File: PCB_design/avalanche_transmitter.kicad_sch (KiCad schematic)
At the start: 22 parts, among them J1 Conn_01x07_Pin, Q1 2N3904, SW1 SW_Push, U1 74HC00

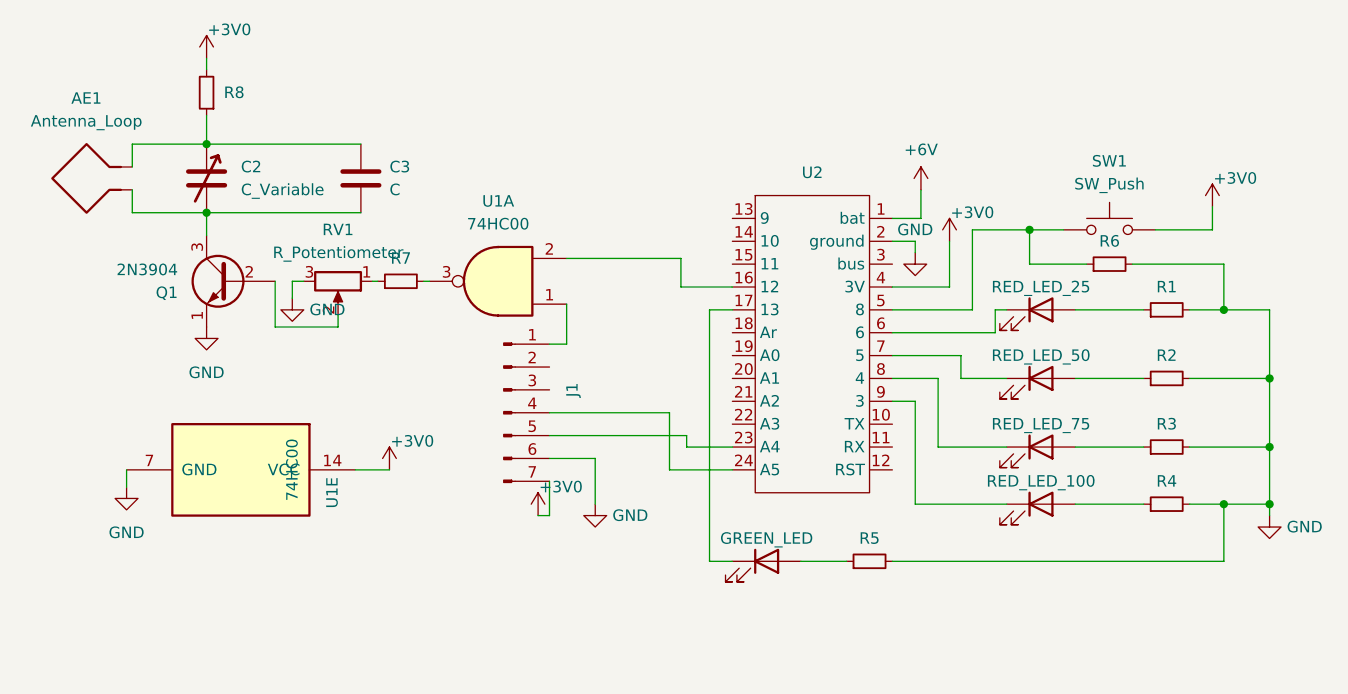
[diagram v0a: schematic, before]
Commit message: Final PCB
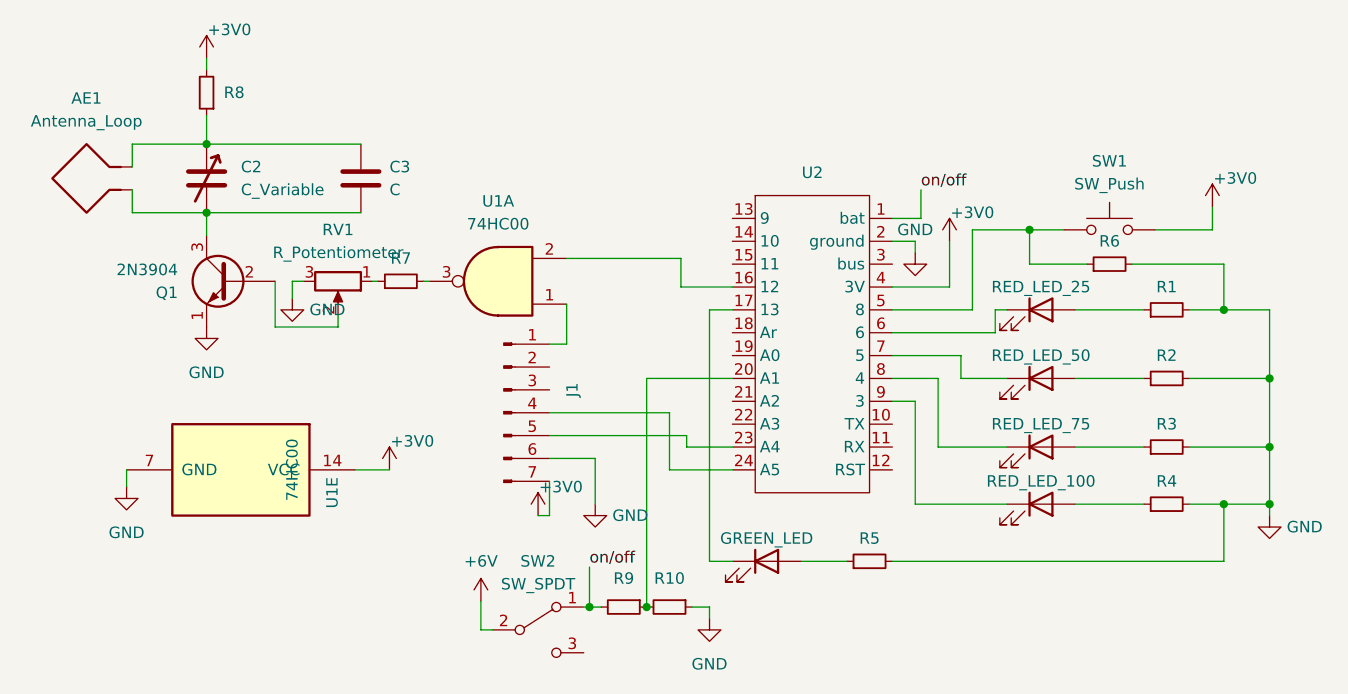
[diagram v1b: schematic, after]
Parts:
- added R10, R9: R_Small, Resistor_THT:R_Axial_DIN0204_L3.6mm_D1.6mm_P7.62mm_Horizontal, symbol Device:R_Small
- added SW2: SW_SPDT, Connector_PinHeader_2.54mm:PinHeader_1x03_P2.54mm_Vertical, symbol Switch:SW_SPDT
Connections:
- net +6V: now also SW2.2 (B); no longer U2.1 (bat)
- net GND: now also R10.1
- net at U2.20 (A1): now also R10.2, R9.1
- new net on/off: R9.2, SW2.1 (A), U2.1 (bat)
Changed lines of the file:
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@@
   (junction (at 196.85 66.04) (diameter 0) (color 0 0 0 0)
   )
+  (junction (at 126.365 77.47) (diameter 0) (color 0 0 0 0)
+  )
   (junction (at 175.26 35.56) (diameter 0) (color 0 0 0 0)
   )
+  (junction (at 132.715 77.47) (diameter 0) (color 0 0 0 0)
+  )
   (junction (at 83.82 26.035) (diameter 0) (color 0 0 0 0)
   )
@@
     (stroke (width 0) (type default))
   )
+  (wire (pts (xy 132.715 52.07) (xy 132.715 77.47))
+    (stroke (width 0) (type default))
+  )
   (wire (pts (xy 167.64 52.07) (xy 167.64 49.53))
     (stroke (width 0) (type default))
@@
     (stroke (width 0) (type default))
   )
+  (wire (pts (xy 126.365 73.025) (xy 126.365 77.47))
+    (stroke (width 0) (type default))
+  )
   (wire (pts (xy 196.85 66.04) (xy 201.93 66.04))
     (stroke (width 0) (type default))
@@
     (stroke (width 0) (type default))
   )
+  (wire (pts (xy 137.795 77.47) (xy 139.7 77.47))
+    (stroke (width 0) (type default))
+  )
   (wire (pts (xy 74.93 62.23) (xy 74.93 64.135))
     (stroke (width 0) (type default))
@@
     (stroke (width 0) (type default))
   )
+  (wire (pts (xy 114.3 76.835) (xy 114.3 80.01))
+    (stroke (width 0) (type default))
+  )
   (wire (pts (xy 136.525 41.91) (xy 142.24 41.91))
     (stroke (width 0) (type default))
@@
     (stroke (width 0) (type default))
   )
+  (wire (pts (xy 142.24 52.07) (xy 132.715 52.07))
+    (stroke (width 0) (type default))
+  )
   (wire (pts (xy 107.95 41.275) (xy 108.585 41.275))
     (stroke (width 0) (type default))
   )
+  (wire (pts (xy 139.7 77.47) (xy 139.7 78.74))
+    (stroke (width 0) (type default))
+  )
   (wire (pts (xy 137.16 59.69) (xy 142.24 59.69))
     (stroke (width 0) (type default))
@@
     (stroke (width 0) (type default))
   )
+  (wire (pts (xy 125.73 77.47) (xy 126.365 77.47))
+    (stroke (width 0) (type default))
+  )
   (wire (pts (xy 171.45 46.99) (xy 160.02 46.99))
     (stroke (width 0) (type default))
@@
     (stroke (width 0) (type default))
   )
+  (wire (pts (xy 114.3 80.01) (xy 115.57 80.01))
+    (stroke (width 0) (type default))
+  )
   (wire (pts (xy 75.565 31.115) (xy 75.565 33.655))
     (stroke (width 0) (type default))
@@
     (stroke (width 0) (type default))
   )
+  (wire (pts (xy 126.365 77.47) (xy 127.635 77.47))
+    (stroke (width 0) (type default))
+  )
   (wire (pts (xy 180.34 44.45) (xy 187.96 44.45))
     (stroke (width 0) (type default))
@@
   (wire (pts (xy 135.255 62.23) (xy 142.24 62.23))
     (stroke (width 0) (type default))
+  )
+  (label "on{slash}off" (at 163.195 31.115 0) (fields_autoplaced)
+    (effects (font (size 1.27 1.27)) (justify left bottom))
+  )
+  (label "on{slash}off" (at 126.365 73.025 0) (fields_autoplaced)
+    (effects (font (size 1.27 1.27)) (justify left bottom))
   )
   (symbol (lib_id "Device:R_Small") (at 83.82 20.32 180) (unit 1)
@@
     )
   )
+  (symbol (lib_id "Switch:SW_SPDT") (at 120.65 80.01 0) (unit 1)
+    (in_bom yes) (on_board yes) (dnp no) (fields_autoplaced)
+    (property "Reference" "SW2" (at 120.65 72.39 0)
+      (effects (font (size 1.27 1.27)))
+    )
+    (property "Value" "SW_SPDT" (at 120.65 74.93 0)
+      (effects (font (size 1.27 1.27)))
+    )
+    (property "Footprint" "Connector_PinHeader_2.54mm:PinHeader_1x03_P2.54mm_Vertical" (at 120.65 80.01 0)
+      (effects (font (size 1.27 1.27)) hide)
+    )
+    (property "Datasheet" "~" (at 120.65 80.01 0)
+      (effects (font (size 1.27 1.27)) hide)
+    )
+    (pin "1")
+    (pin "2")
+    (pin "3")
+    (instances
+      (project "avalanche_transmitter"
+        (path "/8c884e5d-9429-461a-a115-9f5a3e16f11a"
+          (reference "SW2") (unit 1)
+        )
+      )
+    )
+  )
   (symbol (lib_id "power:+3V0") (at 195.58 33.02 0) (unit 1)
     (in_bom yes) (on_board yes) (dnp no)
@@
         (path "/8c884e5d-9429-461a-a115-9f5a3e16f11a"
           (reference "#PWR09") (unit 1)
+        )
+      )
+    )
+  )
+  (symbol (lib_id "power:+6V") (at 114.3 76.835 0) (unit 1)
+    (in_bom yes) (on_board yes) (dnp no) (fields_autoplaced)
+    (property "Reference" "#PWR013" (at 114.3 80.645 0)
+      (effects (font (size 1.27 1.27)) hide)
+    )
+    (property "Value" "+6V" (at 114.3 72.39 0)
+      (effects (font (size 1.27 1.27)))
+    )
+    (property "Footprint" "" (at 114.3 76.835 0)
+      (effects (font (size 1.27 1.27)) hide)
+    )
+    (property "Datasheet" "" (at 114.3 76.835 0)
+      (effects (font (size 1.27 1.27)) hide)
+    )
+    (pin "1")
+    (instances
+      (project "avalanche_transmitter"
+        (path "/8c884e5d-9429-461a-a115-9f5a3e16f11a"
+          (reference "#PWR013") (unit 1)
+        )
+      )
+    )
+  )
+  (symbol (lib_id "Device:R_Small") (at 130.175 77.47 270) (unit 1)
+    (in_bom yes) (on_board yes) (dnp no) (fields_autoplaced)
+    (property "Reference" "R9" (at 130.175 74.295 90)
+      (effects (font (size 1.27 1.27)))
+    )
+    (property "Value" "R_Small" (at 130.175 80.01 90)
+      (effects (font (size 1.27 1.27)) hide)
+    )
+    (property "Footprint" "Resistor_THT:R_Axial_DIN0204_L3.6mm_D1.6mm_P7.62mm_Horizontal" (at 130.175 77.47 0)
+      (effects (font (size 1.27 1.27)) hide)
+    )
+    (property "Datasheet" "~" (at 130.175 77.47 0)
+      (effects (font (size 1.27 1.27)) hide)
+    )
+    (pin "1")
+    (pin "2")
+    (instances
+      (project "avalanche_transmitter"
+        (path "/8c884e5d-9429-461a-a115-9f5a3e16f11a"
+          (reference "R9") (unit 1)
         )
       )
@@
     )
   )
+  (symbol (lib_id "Device:R_Small") (at 135.255 77.47 270) (unit 1)
+    (in_bom yes) (on_board yes) (dnp no) (fields_autoplaced)
+    (property "Reference" "R10" (at 135.255 74.295 90)
+      (effects (font (size 1.27 1.27)))
+    )
+    (property "Value" "R_Small" (at 135.255 80.01 90)
+      (effects (font (size 1.27 1.27)) hide)
+    )
+    (property "Footprint" "Resistor_THT:R_Axial_DIN0204_L3.6mm_D1.6mm_P7.62mm_Horizontal" (at 135.255 77.47 0)
+      (effects (font (size 1.27 1.27)) hide)
+    )
+    (property "Datasheet" "~" (at 135.255 77.47 0)
+      (effects (font (size 1.27 1.27)) hide)
+    )
+    (pin "1")
+    (pin "2")
+    (instances
+      (project "avalanche_transmitter"
+        (path "/8c884e5d-9429-461a-a115-9f5a3e16f11a"
+          (reference "R10") (unit 1)
+        )
+      )
+    )
+  )
   (symbol (lib_id "Device:R_Small") (at 190.5 52.07 90) (unit 1)
     (in_bom yes) (on_board yes) (dnp no) (fields_autoplaced)
@@
         (path "/8c884e5d-9429-461a-a115-9f5a3e16f11a"
           (reference "R2") (unit 1)
+        )
+      )
+    )
+  )
+  (symbol (lib_id "power:GND") (at 139.7 78.74 0) (unit 1)
+    (in_bom yes) (on_board yes) (dnp no) (fields_autoplaced)
+    (property "Reference" "#PWR014" (at 139.7 85.09 0)
+      (effects (font (size 1.27 1.27)) hide)
+    )
+    (property "Value" "GND" (at 139.7 83.82 0)
+      (effects (font (size 1.27 1.27)))
+    )
+    (property "Footprint" "" (at 139.7 78.74 0)
+      (effects (font (size 1.27 1.27)) hide)
+    )
+    (property "Datasheet" "" (at 139.7 78.74 0)
+      (effects (font (size 1.27 1.27)) hide)
+    )
+    (pin "1")
+    (instances
+      (project "avalanche_transmitter"
+        (path "/8c884e5d-9429-461a-a115-9f5a3e16f11a"
+          (reference "#PWR014") (unit 1)
         )
       )
@@
         )
       )
-    )
-  )
-  (symbol (lib_id "power:+6V") (at 163.195 31.115 0) (unit 1)
-    (in_bom yes) (on_board yes) (dnp no) (fields_autoplaced)
-    (property "Reference" "#PWR06" (at 163.195 34.925 0)
-      (effects (font (size 1.27 1.27)) hide)
-    )
-    (property "Value" "+6V" (at 163.195 26.67 0)
-      (effects (font (size 1.27 1.27)))
-    )
-    (property "Footprint" "" (at 163.195 31.115 0)
-      (effects (font (size 1.27 1.27)) hide)
-    )
-    (property "Datasheet" "" (at 163.195 31.115 0)
-      (effects (font (size 1.27 1.27)) hide)
-    )
-    (pin "1")
-    (instances
-      (project "avalanche_transmitter"
-        (path "/8c884e5d-9429-461a-a115-9f5a3e16f11a"
-          (reference "#PWR06") (unit 1)
-        )
-      )
